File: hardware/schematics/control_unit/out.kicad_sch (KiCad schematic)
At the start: 93 parts, among them K1 Relay_SPDT, K2 Relay_SPDT, K3 Relay_SPDT, K4 Relay_SPDT, K5 Relay_SPDT, Q1 2N7000, Q10 IRFZ44N, Q11 2N7000, Q12 IRFZ44N, Q13 IRFZ44N, Q14 IRFZ44N, Q15 IRFZ44N, Q16 IRFZ44N, Q17 IRFZ44N, Q2 2N7000, Q3 IRFZ44N, Q4 IRFZ44N, Q5 IRFZ44N, Q6 2N7000, Q7 2N7000, Q8 IRFZ44N, Q9 IRFZ44N, U1 PC817, U10 PC817, U11 PC817, U12 PC817, U2 PC817, U3 PC817, U4 PC817, U5 PC817, U6 PC817, U7 PC817, U8 PC817, U9 PC817

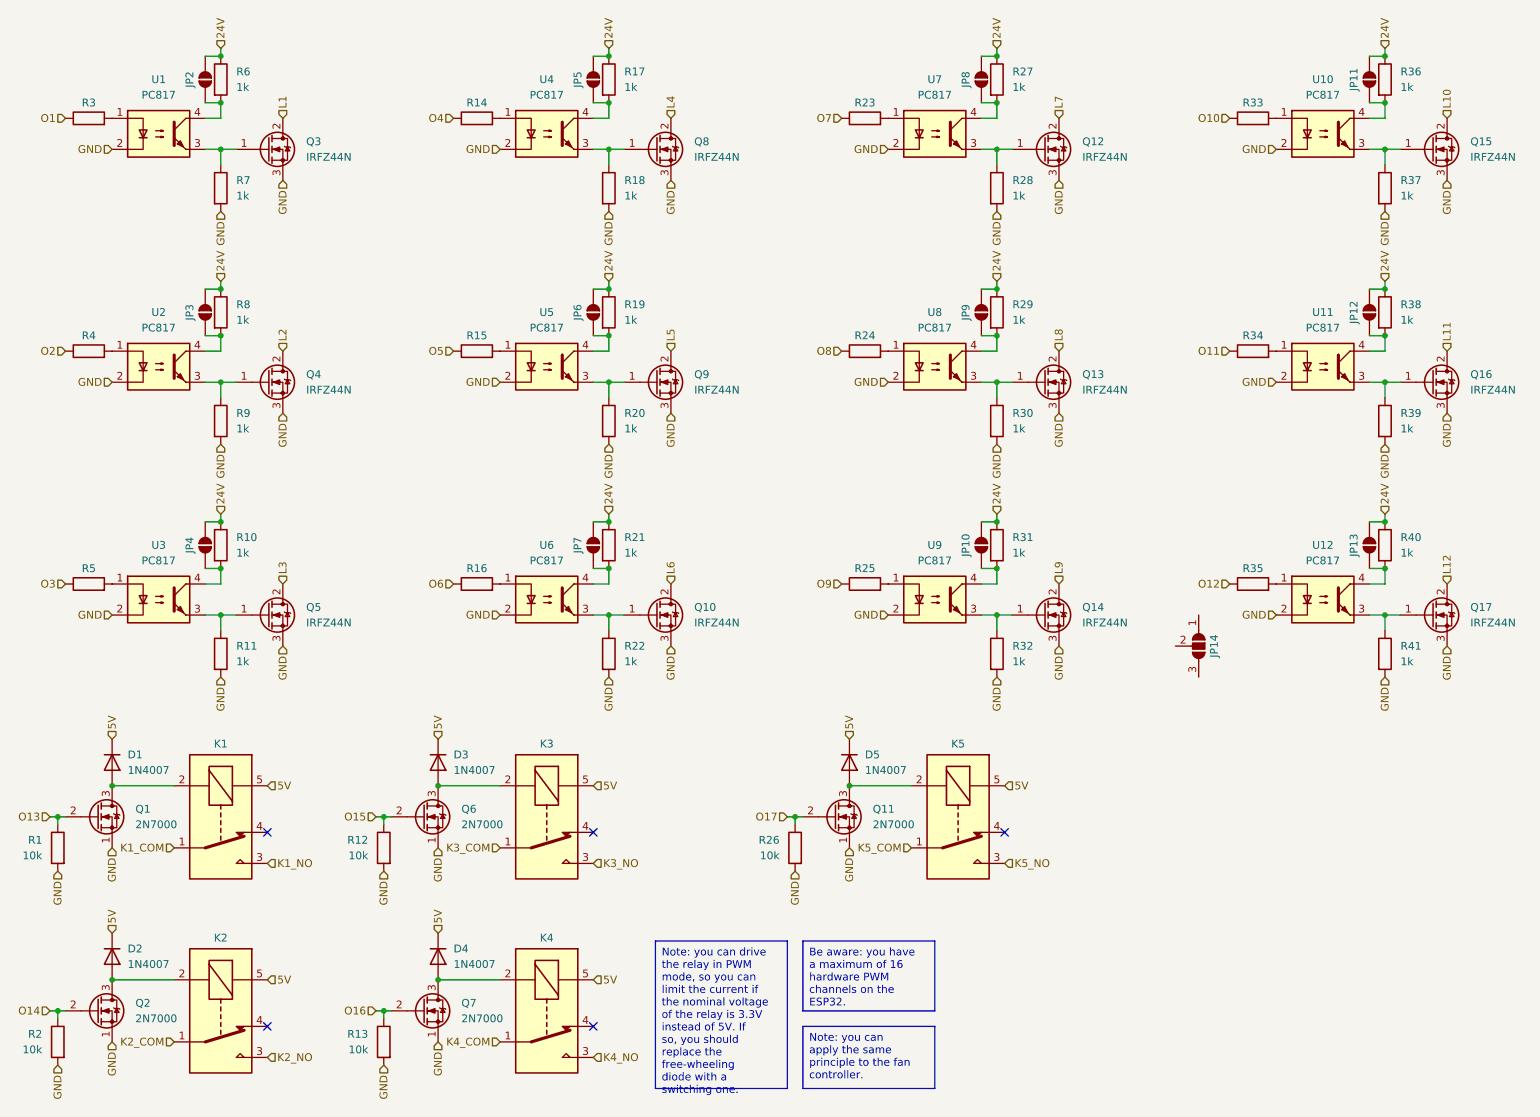
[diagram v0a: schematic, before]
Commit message: feat
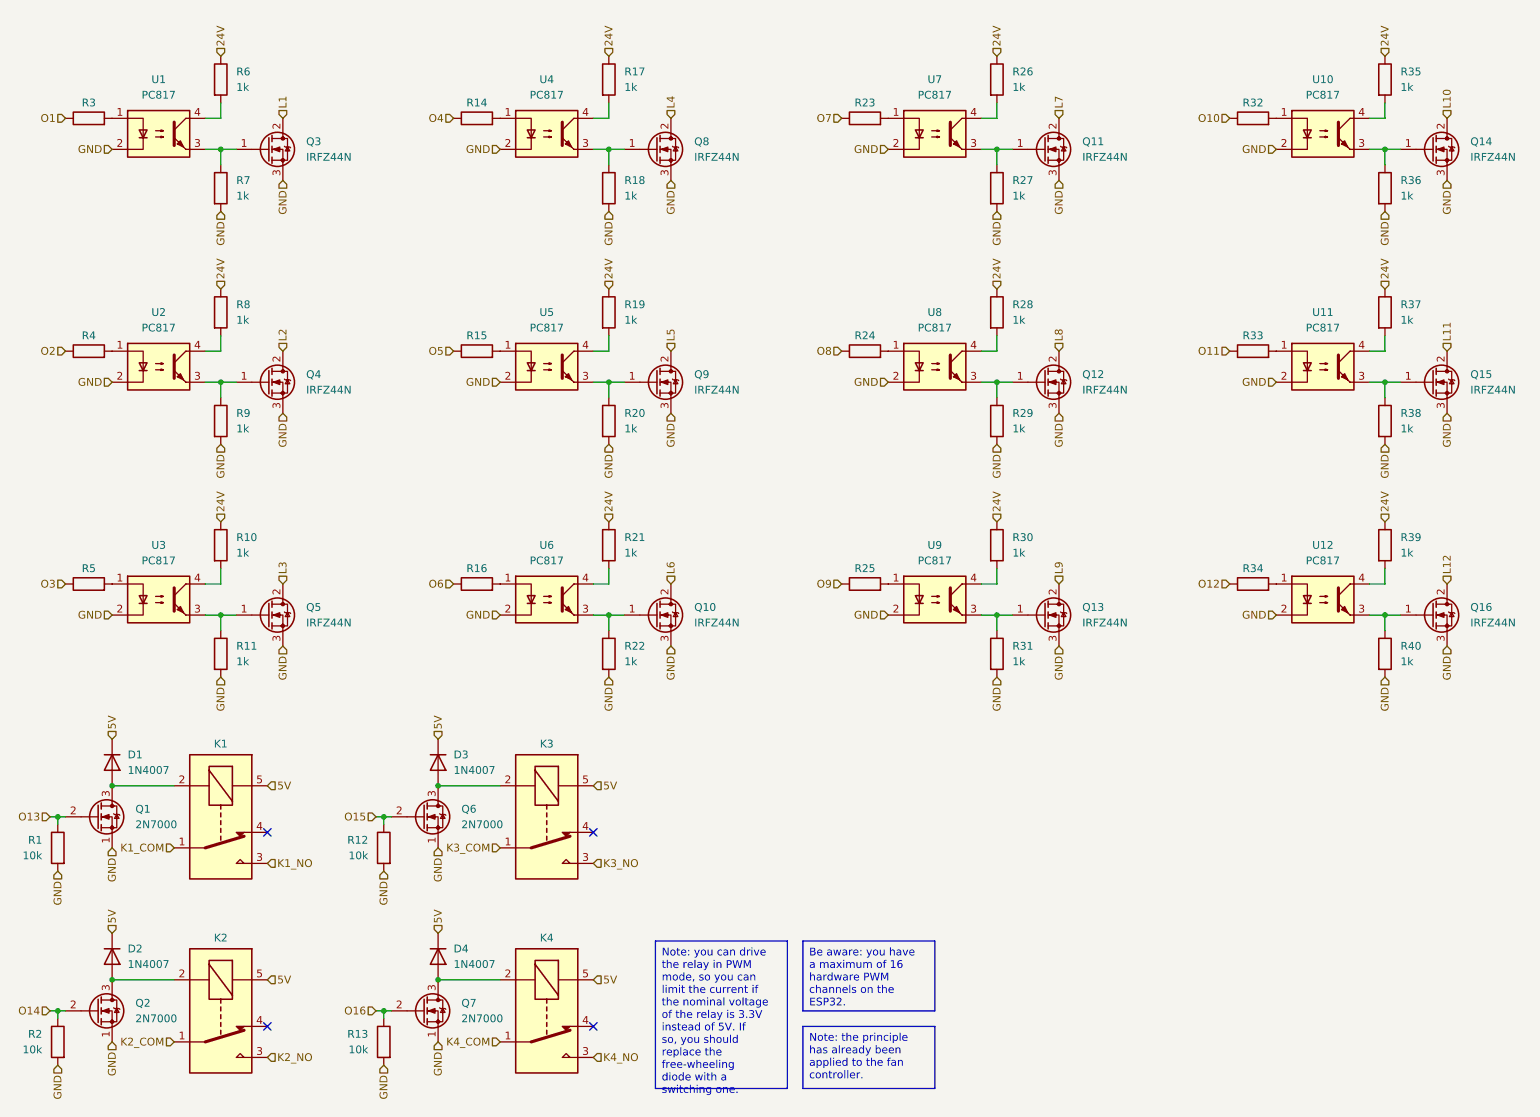
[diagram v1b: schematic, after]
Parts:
- removed D5: 1N4007, Diode_THT:D_DO-41_SOD81_P2.54mm_Vertical_KathodeUp, symbol Diode:1N4007
- removed JP10, JP11, JP12, JP13, JP2, JP3, JP4, JP5, JP6, JP7, JP8, JP9: SolderJumper_2_Open, symbol Jumper:SolderJumper_2_Open
- removed JP14: (no value), Jumper:SolderJumper-3_P1.3mm_Open_Pad1.0x1.5mm, symbol Jumper:SolderJumper_3_Open
- removed K5: Relay_SPDT, Relay_THT:Relay_SPDT_Omron-G5LE-1, symbol Relay:Relay_SPDT
- removed Q11: 2N7000, Package_TO_SOT_THT:TO-92_Inline, symbol Transistor_FET:2N7000
- removed R26: 10k, symbol Device:R
- R1, R10, R11, R12, R13, R14, R15, R16, R17, R18, R19, R2, R20, R21, R22, R23, R24, R25, R3, R4, R5, R6, R7, R8, R9: footprint (none) -> Resistor_THT:R_Axial_DIN0207_L6.3mm_D2.5mm_P7.62mm_Horizontal
- R26: renamed from R27; footprint (none) -> Resistor_THT:R_Axial_DIN0207_L6.3mm_D2.5mm_P7.62mm_Horizontal
- R27: renamed from R28; footprint (none) -> Resistor_THT:R_Axial_DIN0207_L6.3mm_D2.5mm_P7.62mm_Horizontal
- R28: renamed from R29; footprint (none) -> Resistor_THT:R_Axial_DIN0207_L6.3mm_D2.5mm_P7.62mm_Horizontal
- R29: renamed from R30; footprint (none) -> Resistor_THT:R_Axial_DIN0207_L6.3mm_D2.5mm_P7.62mm_Horizontal
- R30: renamed from R31; footprint (none) -> Resistor_THT:R_Axial_DIN0207_L6.3mm_D2.5mm_P7.62mm_Horizontal
- R31: renamed from R32; footprint (none) -> Resistor_THT:R_Axial_DIN0207_L6.3mm_D2.5mm_P7.62mm_Horizontal
- R32: renamed from R33; footprint (none) -> Resistor_THT:R_Axial_DIN0207_L6.3mm_D2.5mm_P7.62mm_Horizontal
- R33: renamed from R34; footprint (none) -> Resistor_THT:R_Axial_DIN0207_L6.3mm_D2.5mm_P7.62mm_Horizontal
- R34: renamed from R35; footprint (none) -> Resistor_THT:R_Axial_DIN0207_L6.3mm_D2.5mm_P7.62mm_Horizontal
- R35: renamed from R36; footprint (none) -> Resistor_THT:R_Axial_DIN0207_L6.3mm_D2.5mm_P7.62mm_Horizontal
- R36: renamed from R37; footprint (none) -> Resistor_THT:R_Axial_DIN0207_L6.3mm_D2.5mm_P7.62mm_Horizontal
- R37: renamed from R38; footprint (none) -> Resistor_THT:R_Axial_DIN0207_L6.3mm_D2.5mm_P7.62mm_Horizontal
- R38: renamed from R39; footprint (none) -> Resistor_THT:R_Axial_DIN0207_L6.3mm_D2.5mm_P7.62mm_Horizontal
- R39: renamed from R40; footprint (none) -> Resistor_THT:R_Axial_DIN0207_L6.3mm_D2.5mm_P7.62mm_Horizontal
- R40: renamed from R41; footprint (none) -> Resistor_THT:R_Axial_DIN0207_L6.3mm_D2.5mm_P7.62mm_Horizontal
- renumbered Q12 to Q11, Q13 to Q12, Q14 to Q13, Q15 to Q14, Q16 to Q15, Q17 to Q16
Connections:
- no-connect marks 5 -> 4

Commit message: !feat
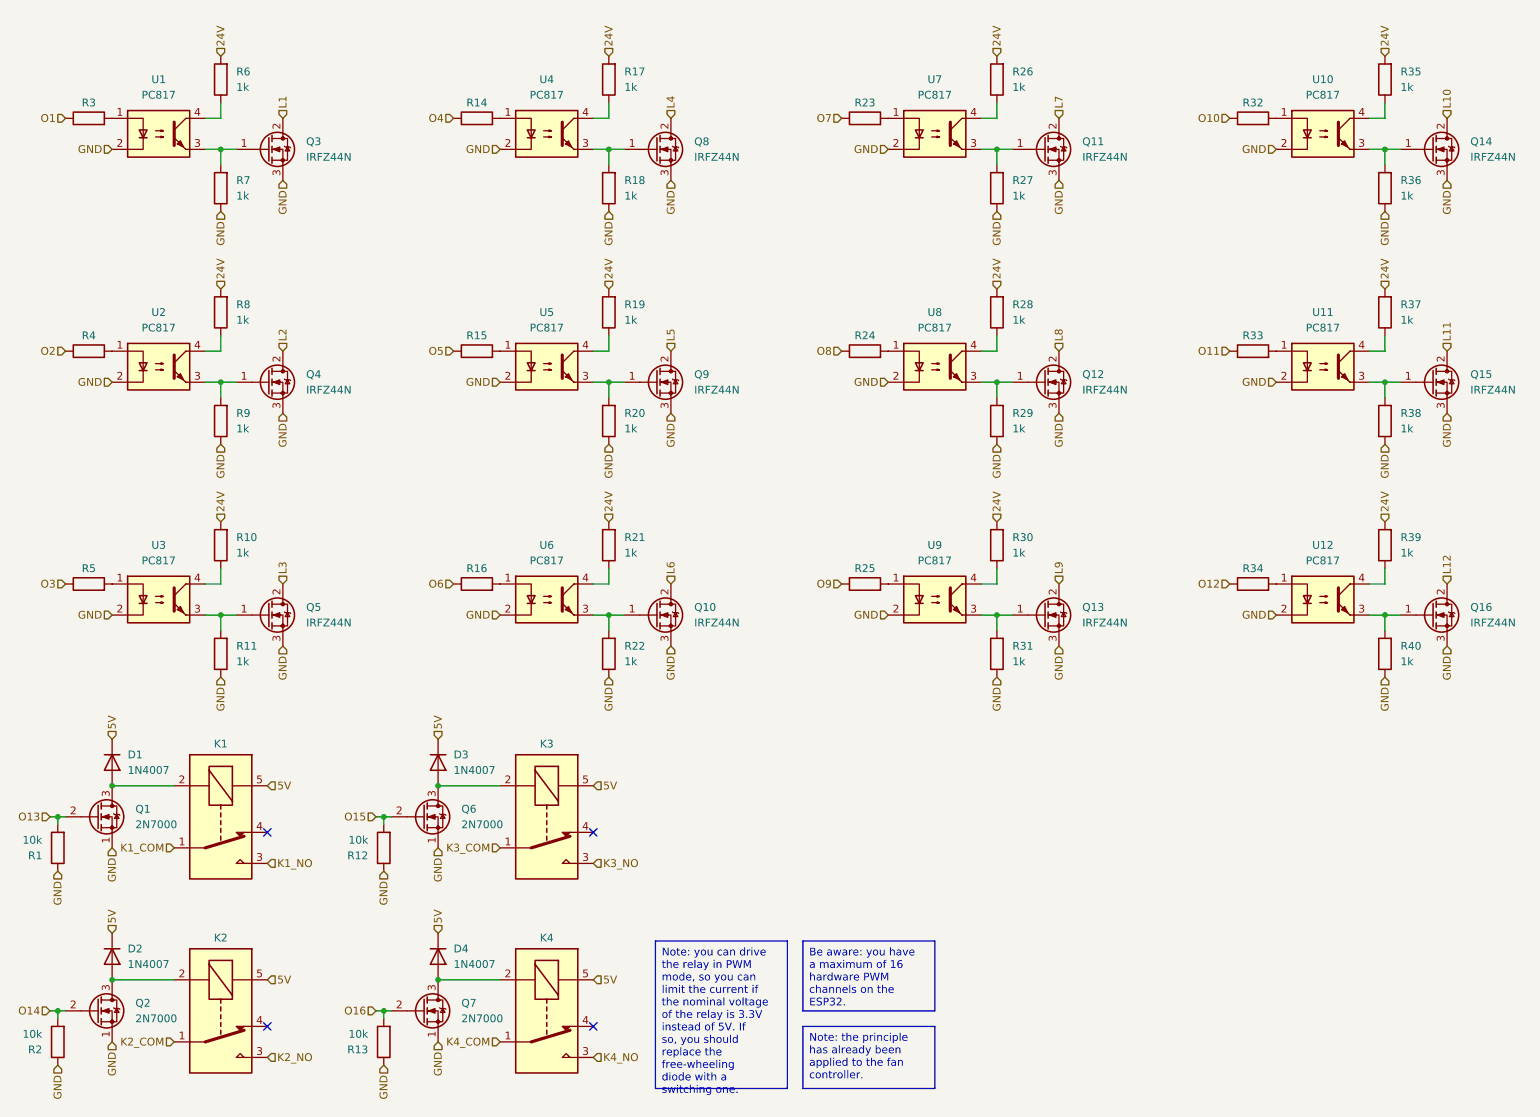
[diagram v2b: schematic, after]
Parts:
- D1, D2, D3, D4: footprint Diode_THT:D_DO-41_SOD81_P2.54mm_Vertical_KathodeUp -> Diode_THT:D_DO-41_SOD81_P7.62mm_Horizontal
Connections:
- net 24V: now also R10.2, R17.2, R19.2, R21.2, R26.2, R28.2, R30.2, R35.2, R37.2, R39.2, R6.2, R8.2; no longer R10.1, R17.1, R19.1, R21.1, R26.1, R28.1, R30.1, R35.1, R37.1, R39.1, R6.1, R8.1
- net GND: now also R1.1, R11.1, R12.1, R13.1, R18.1, R2.1, R20.1, R22.1, R27.1, R29.1, R31.1, R36.1, R38.1, R40.1, R7.1, R9.1; no longer R1.2, R11.2, R12.2, R13.2, R18.2, R2.2, R20.2, R22.2, R27.2, R29.2, R31.2, R36.2, R38.2, R40.2, R7.2, R9.2
- net O13: now also R1.2; no longer R1.1
- net O14: now also R2.2; no longer R2.1
- net O15: now also R12.2; no longer R12.1
- net O16: now also R13.2; no longer R13.1
- net at U2.4: now also R8.1; no longer R8.2
- net at Q9.1 (G), U5.3: now also R20.2; no longer R20.1
- net at Q15.1 (G), U11.3: now also R38.2; no longer R38.1
- net at U10.4: now also R35.1; no longer R35.2
- net at U3.4: now also R10.1; no longer R10.2
- net at Q5.1 (G), U3.3: now also R11.2; no longer R11.1
- net at U9.4: now also R30.1; no longer R30.2
- net at Q4.1 (G), U2.3: now also R9.2; no longer R9.1
- net at Q3.1 (G), U1.3: now also R7.2; no longer R7.1
- net at U11.4: now also R37.1; no longer R37.2
- net at U7.4: now also R26.1; no longer R26.2
- net at Q13.1 (G), U9.3: now also R31.2; no longer R31.1
- net at Q11.1 (G), U7.3: now also R27.2; no longer R27.1
- net at Q14.1 (G), U10.3: now also R36.2; no longer R36.1
- net at Q8.1 (G), U4.3: now also R18.2; no longer R18.1
- net at U4.4: now also R17.1; no longer R17.2
- net at Q10.1 (G), U6.3: now also R22.2; no longer R22.1
- net at U6.4: now also R21.1; no longer R21.2
- net at U5.4: now also R19.1; no longer R19.2
- net at U1.4: now also R6.1; no longer R6.2
- net at U8.4: now also R28.1; no longer R28.2
- net at Q12.1 (G), U8.3: now also R29.2; no longer R29.1
- net at Q16.1 (G), U12.3: now also R40.2; no longer R40.1
- net at U12.4: now also R39.1; no longer R39.2
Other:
- moved on the sheet: R1, R10, R11, R12, R13, R17, R18, R19, R2, R20, R21, R22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
